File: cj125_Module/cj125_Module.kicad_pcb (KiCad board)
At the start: 2 copper layers, 56 x 22 mm, 32 parts, among them J1 Conn_02x20_Odd_Even, Q1 buk 100-50, U1 TS5A3166DCKR, U2 TS5A3166DCKR, U3 CJ125

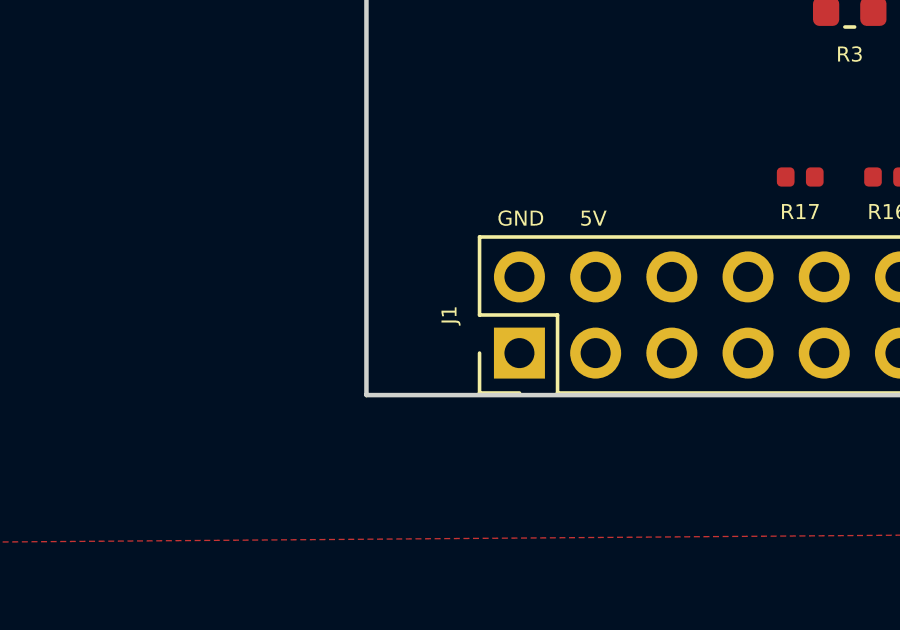
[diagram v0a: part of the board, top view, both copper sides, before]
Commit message: draft
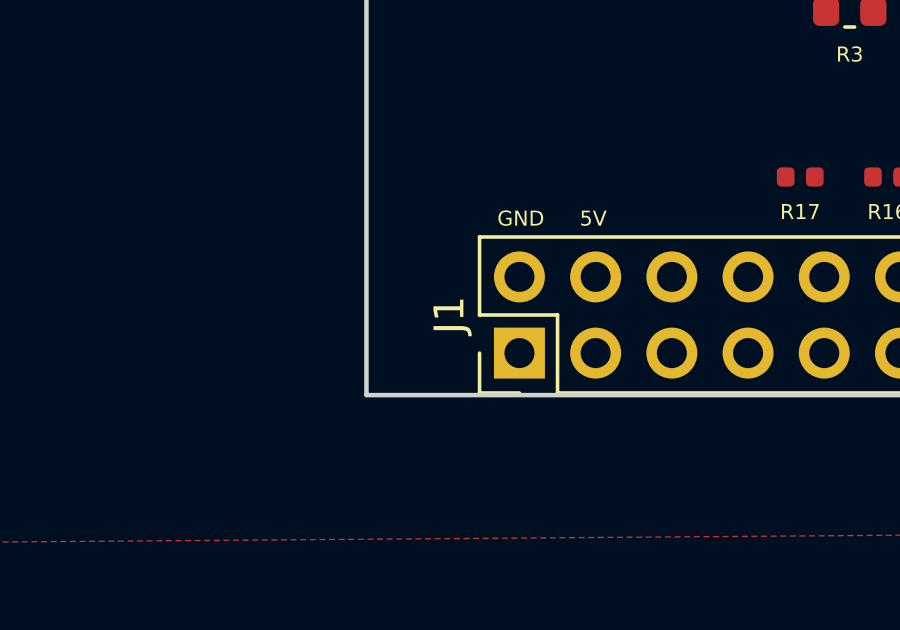
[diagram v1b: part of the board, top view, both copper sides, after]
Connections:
- U3 pad 13: /CJ125-1-SCK -> (no net)
- U3 pad 15: /CJ125-1-SI -> (no net)
- U3 pad 17: /CJ125-1-SS -> (no net)
